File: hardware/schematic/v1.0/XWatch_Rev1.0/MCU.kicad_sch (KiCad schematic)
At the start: 24 parts, among them U1 STM32L4R9AII6U, X1 NX3215SA_32_768KHZ_EXS00A-MU0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, X2 TXM16M0004252CBCEO00T

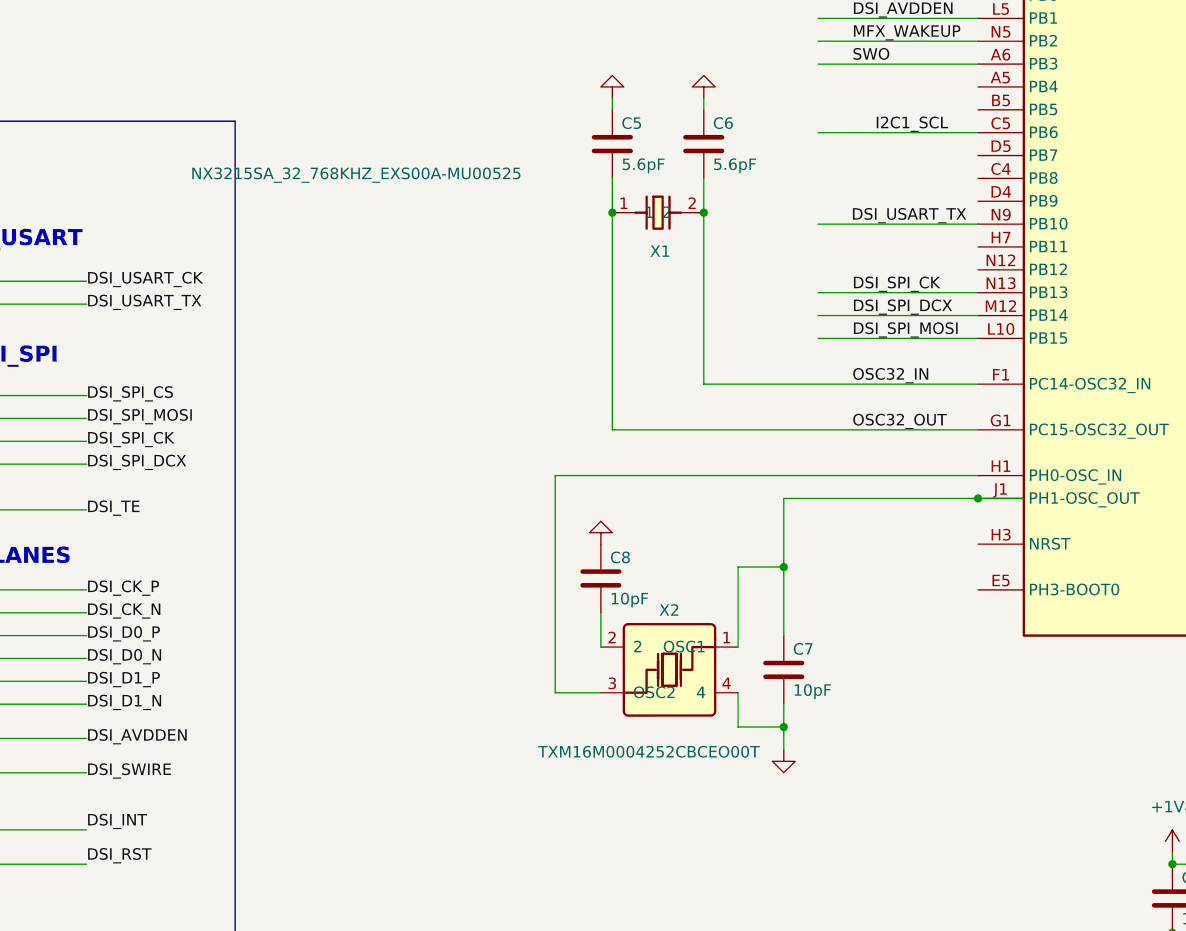
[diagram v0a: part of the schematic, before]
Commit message: add rev2.0
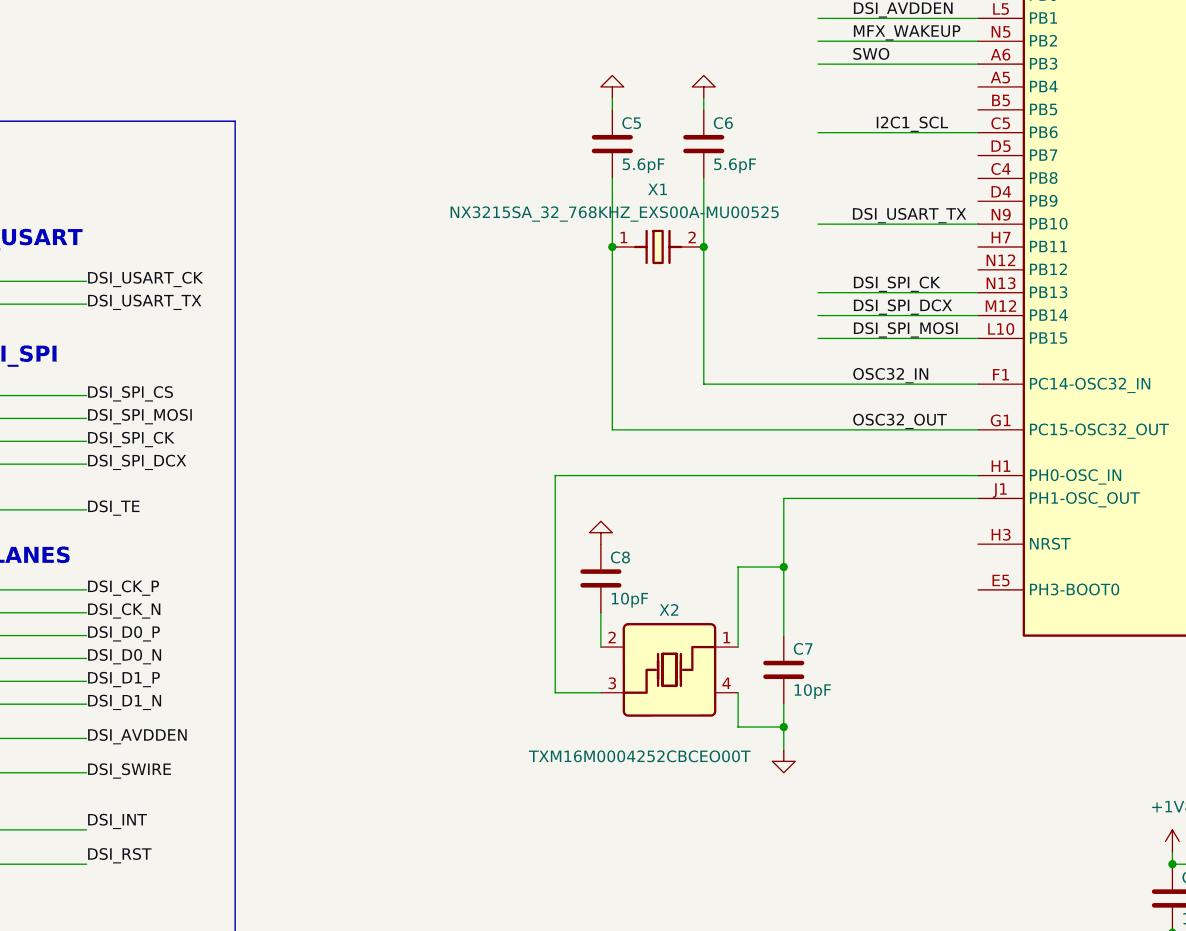
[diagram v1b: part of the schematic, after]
